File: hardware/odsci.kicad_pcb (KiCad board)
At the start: 4 copper layers, 50 x 69.2 mm, 35 parts, among them J1 USB_C_Receptacle, J2 Conn_01x03_Pin, J3 Conn_01x04_Pin, J4 Screw_Terminal_01x03, SW1 SW_Push, U1 TPS7A4701xRGW, U2 STM32F042K6Tx, U3 USBLC6-2SC6

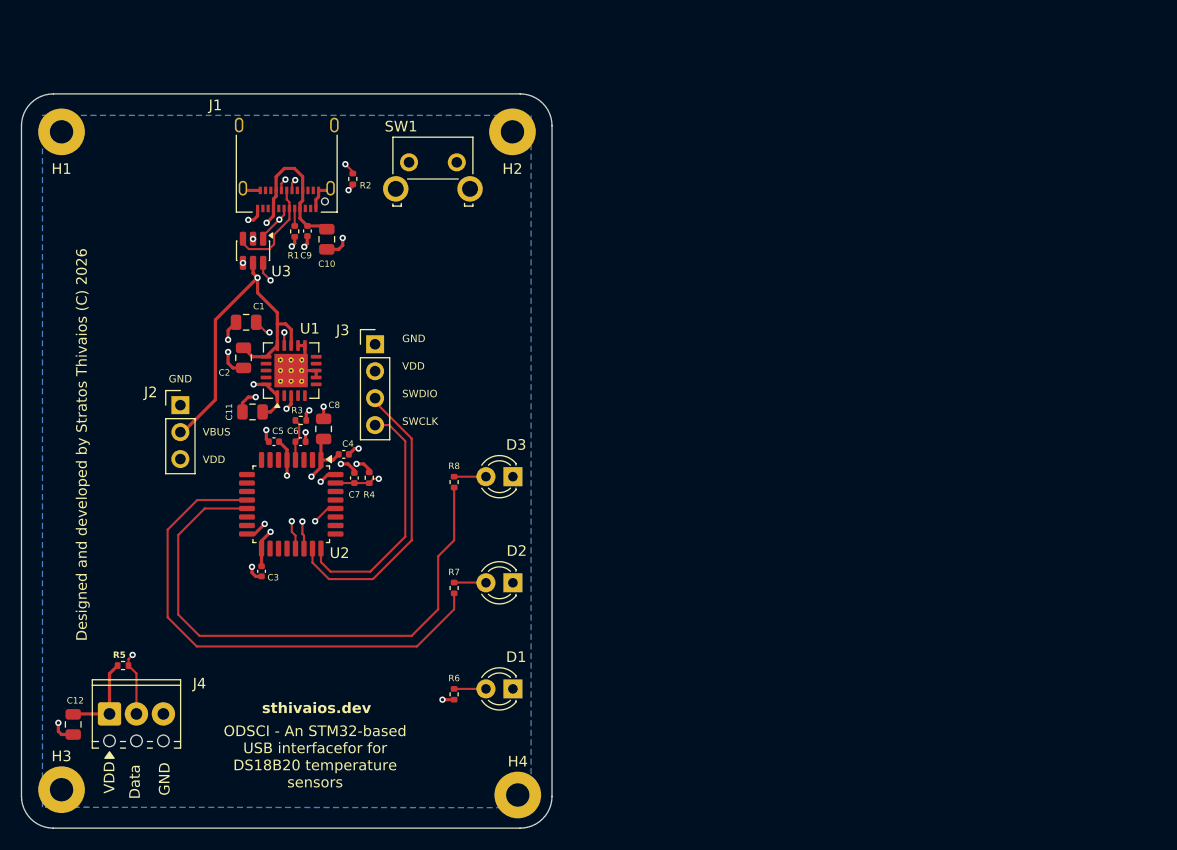
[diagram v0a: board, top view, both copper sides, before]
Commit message: hardware: layout of pcb
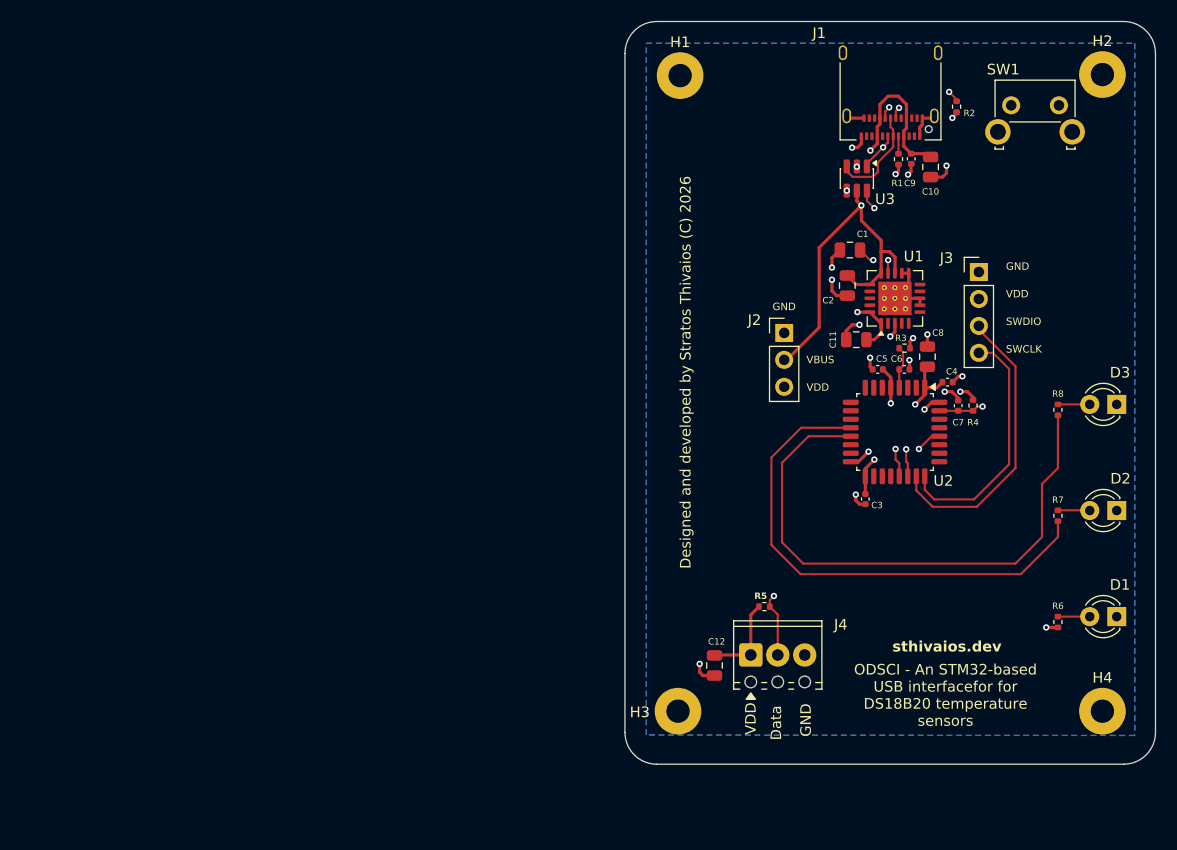
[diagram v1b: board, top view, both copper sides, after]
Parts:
- moved C12 60.7 mm to (191.0, 125.8)
- moved J4 60.7 mm to (194.5, 124.8)
- moved R5 60.7 mm to (195.7, 120.2)
- moved H3 58.6 mm to (187.6, 130.1)
- moved H1 58.5 mm to (187.8, 70.2)
- moved C1 57.3 mm to (203.8, 86.6)
- moved C10 57.3 mm to (211.4, 78.8)
- moved C11 57.3 mm to (204.4, 95.1)
- moved C2 57.3 mm to (203.6, 90.0)
- moved C3 57.3 mm to (205.3, 110.1)
- moved C4 57.3 mm to (213.0, 99.1)
- moved C5 57.3 mm to (206.4, 97.9)
- moved C6 57.3 mm to (208.9, 97.9)
- moved C7 57.3 mm to (214.0, 101.3)
- moved C8 57.3 mm to (211.1, 96.7)
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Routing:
- net ONEWIRE_BUS: track 37.8 -> 34.0 mm
- net Net-(U2-PB8): track 37.1 -> 35.6 mm
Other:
- board size 50 x 69.2 mm -> 50 x 70 mm
